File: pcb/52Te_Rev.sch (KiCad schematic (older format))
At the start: 56 parts, among them J1 MJ-4PP-9, J2 Conn_01x04, SW1 SW_PUSH, SW10 SW_PUSH, SW11 SW_PUSH, SW12 SW_PUSH, SW13 SW_PUSH, SW14 SW_PUSH, SW15 SW_PUSH, SW16 SW_PUSH, SW17 SW_PUSH, SW18 SW_PUSH, SW19 SW_PUSH, SW2 SW_PUSH, SW20 SW_PUSH, SW21 SW_PUSH, SW22 SW_PUSH, SW23 SW_PUSH, SW24 SW_PUSH, SW25 SW_PUSH, SW26 SW_PUSH, SW27 SW_PUSH, SW3 SW_PUSH, SW4 SW_PUSH, SW5 SW_PUSH, SW6 SW_PUSH, SW7 SW_PUSH, SW8 SW_PUSH, SW9 SW_PUSH, U1 ProMicro

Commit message: removed OLED footprints
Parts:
- removed J2: Conn_01x04, kbd:OLED, symbol Connector_Generic:Conn_01x04
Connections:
- wire segments 77 -> 69
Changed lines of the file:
@@
 Wire Wire Line
 	5650 1750 6550 1750
-$Comp
-L Connector_Generic:Conn_01x04 J2
-U 1 1 5C51C912
-P 9150 4150
-F 0 "J2" H 9230 4142 50  0000 L CNN
-F 1 "Conn_01x04" H 9230 4051 50  0000 L CNN
-F 2 "kbd:OLED" H 9150 4150 50  0001 C CNN
-F 3 "~" H 9150 4150 50  0001 C CNN
-	1    9150 4150
-	1    0    0    -1
-$EndComp
-$Comp
-L Atreus62-cache:GND #PWR09
-U 1 1 5C51CC2A
-P 8600 4050
-F 0 "#PWR09" H 8600 3800 50  0001 C CNN
-F 1 "GND" V 8605 3922 50  0000 R CNN
-F 2 "" H 8600 4050 50  0000 C CNN
-F 3 "" H 8600 4050 50  0000 C CNN
-	1    8600 4050
-	0    1    1    0
-$EndComp
-$Comp
-L Atreus62-cache:VCC #PWR010
-U 1 1 5C51CD02
-P 8600 4150
-F 0 "#PWR010" H 8600 4000 50  0001 C CNN
-F 1 "VCC" V 8618 4277 50  0000 L CNN
-F 2 "" H 8600 4150 50  0000 C CNN
-F 3 "" H 8600 4150 50  0000 C CNN
-	1    8600 4150
-	0    -1   -1   0
-$EndComp
-Wire Wire Line
-	8950 4050 8600 4050
-Wire Wire Line
-	8950 4150 8600 4150
-Wire Wire Line
-	8950 4250 8650 4250
-Wire Wire Line
-	8650 4250 8650 4350
-Wire Wire Line
-	8450 4350 8650 4350
-Text GLabel 8450 4350 0    50   Input ~ 0
-SCL
-Wire Wire Line
-	8950 4350 8700 4350
-Wire Wire Line
-	8700 4350 8700 4500
-Wire Wire Line
-	8700 4500 8450 4500
-Text GLabel 8450 4500 0    50   Input ~ 0
-SDA
 NoConn ~ 7750 2050
 Wire Wire Line

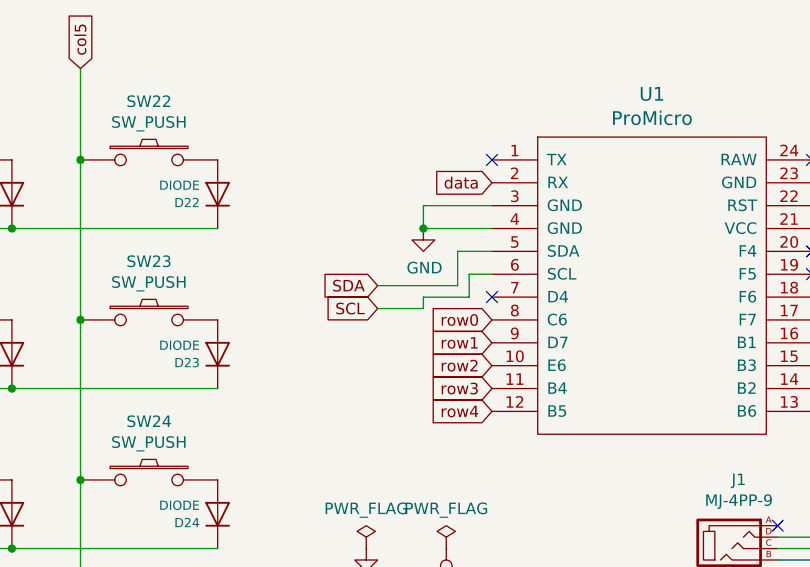
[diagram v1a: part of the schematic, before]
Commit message: new gerber file
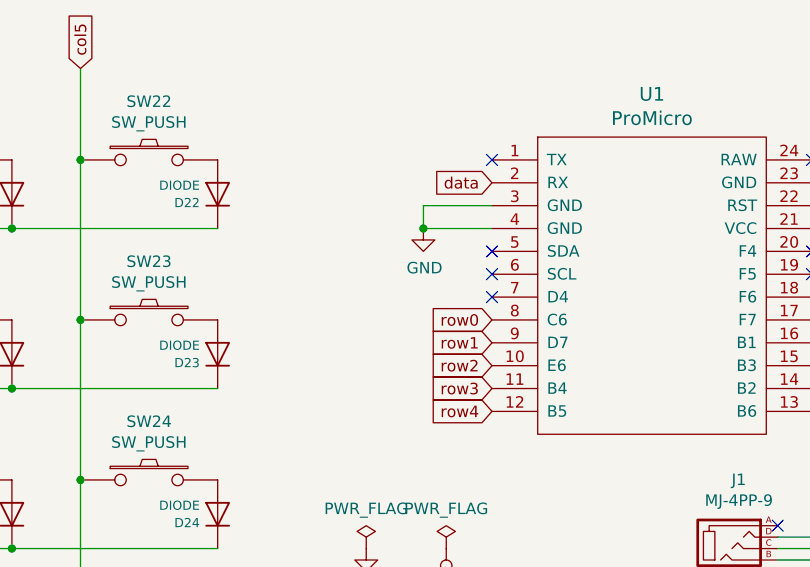
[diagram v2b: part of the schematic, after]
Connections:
- net SCL: no longer names the net of U1.6 (SCL)
- net SDA: no longer names the net of U1.5 (SDA)
- no-connect marks 6 -> 8
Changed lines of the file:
@@
 EESchema Schematic File Version 4
 LIBS:52Te_Rev-cache
-EELAYER 26 0
+EELAYER 29 0
 EELAYER END
 $Descr A4 11693 8268
@@
 NoConn ~ 7750 2050
 Wire Wire Line
-	7750 1850 7600 1850
-Wire Wire Line
-	7600 1850 7600 2000
-Wire Wire Line
-	7250 2000 7600 2000
-Wire Wire Line
-	7750 1950 7650 1950
-Wire Wire Line
-	7650 1950 7650 2050
-Wire Wire Line
-	7650 2050 7450 2050
-Wire Wire Line
-	7450 2050 7450 2100
-Wire Wire Line
-	7450 2100 7250 2100
-Text GLabel 7250 2000 0    50   Input ~ 0
-SDA
-Text GLabel 7250 2100 0    50   Input ~ 0
-SCL
-Wire Wire Line
 	9000 3150 9150 3150
 Wire Wire Line
@@
 Wire Wire Line
 	9000 3200 9500 3200
+NoConn ~ 7750 1850
+NoConn ~ 7750 1950
 $EndSCHEMATC
